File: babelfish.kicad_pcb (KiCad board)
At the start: 2 copper layers, 56 x 38.2 mm, 88 parts, among them J1 Conn_02x02_Odd_Even, J2 SWD, J3 DE9 Female, J4 USB_A, Q1 BSS138, SW1 TS342A2P-WZ, SW2 TS342A2P-WZ, SW3 SK12D07VG5_C3020419, U1 RP2040, U10 74HC4052PW,118, U11 MAX3232IDR, U2 TPS2113ADRBR, U3 GT-USB-7010ASV, U4 W25Q128JVS, U5 TPMCP1703T-5002E_CB, U6 TPMCP1703T-3302E_CB, U7 74HC4052PW,118, U8 74HC4052PW,118, U9 74HC4052PW,118, X1 X322512MSB4SI

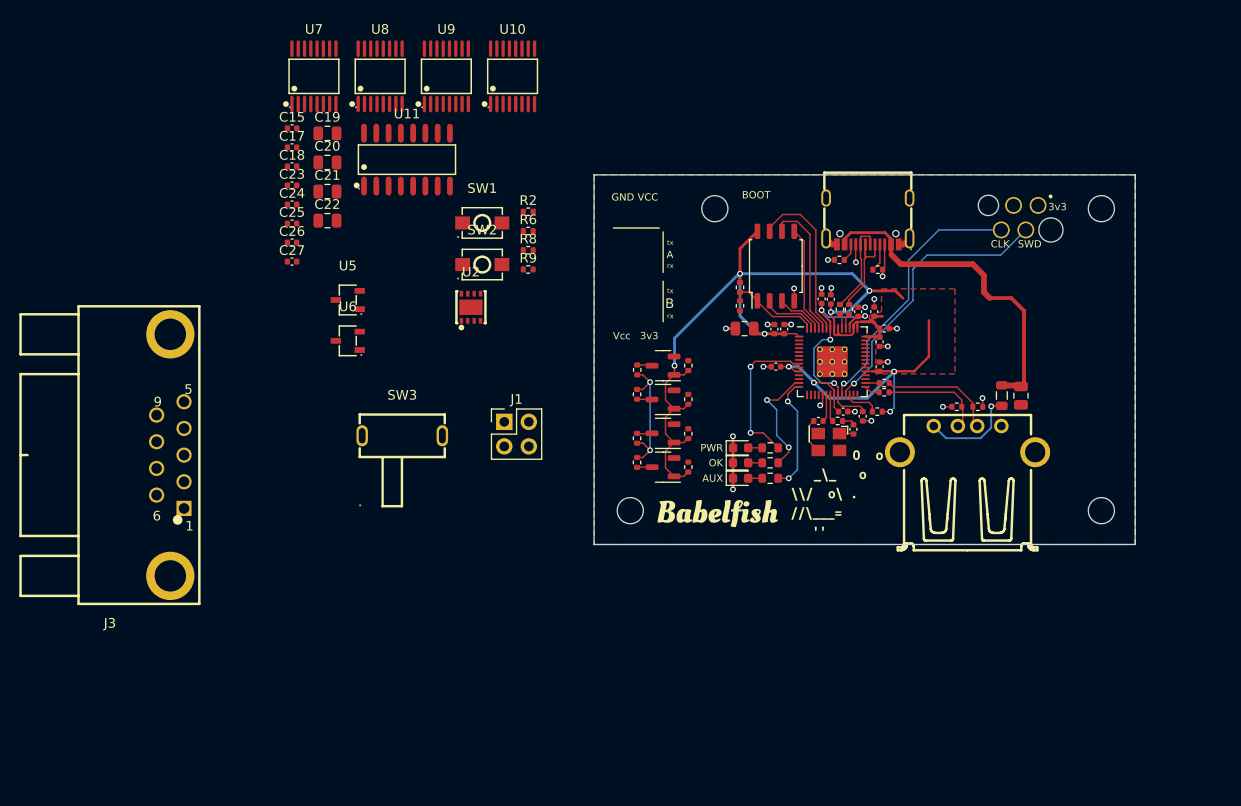
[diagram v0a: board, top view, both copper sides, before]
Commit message: Layout v2 done
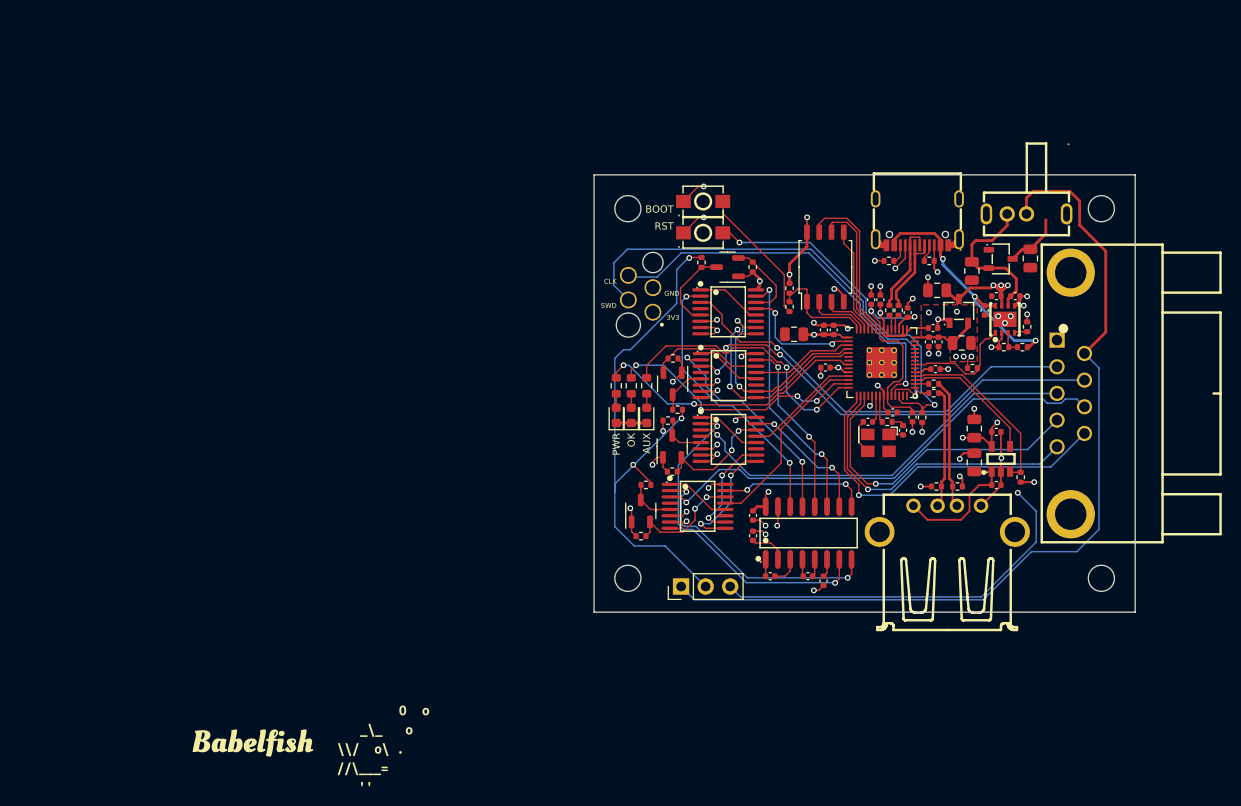
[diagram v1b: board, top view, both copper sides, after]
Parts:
- removed FB1: FerriteBead_Small, Inductor_SMD:L_0805_2012Metric
- added C29: 10u, Capacitor_SMD:C_0805_2012Metric, F.Cu at (121.6, 99.2)
- added C30: 100n, Capacitor_SMD:C_0402_1005Metric, F.Cu at (123.9, 96.1)
- added C31: 10u, Capacitor_SMD:C_0805_2012Metric, F.Cu at (121.6, 95.8)
- added R28: 10k, Resistor_SMD:R_0402_1005Metric, F.Cu at (126.4, 100.8)
- added U12: AP2191WG-7, lcsc:SOT-25-5_L2.9-W1.6-P0.95-LS2.8-BL, F.Cu at (124.4, 98.9)
- C28: value 10u -> 100n; footprint Capacitor_SMD:C_0805_2012Metric -> Capacitor_SMD:C_0402_1005Metric
- J1: value Conn_02x02_Odd_Even -> Shifter Power; footprint Connector_PinHeader_2.54mm:PinHeader_2x02_P2.54mm_Vertical -> Connector_PinHeader_2.54mm:PinHeader_1x03_P2.54mm_Vertical
- moved J3 93.4 mm to (131.6, 92.1), turned to 0 degrees
- moved C18 76.0 mm to (125.8, 82.1)
- moved C17 74.5 mm to (123.9, 82.1), turned to 180 degrees
- moved C15 74.1 mm to (122.7, 83.5), turned to -90 degrees
- moved C19 73.9 mm to (127.4, 78.2), turned to -90 degrees
- moved SW3 68.6 mm to (127.0, 73.5), turned to 180 degrees
- moved U5 67.7 mm to (124.3, 78.2), turned to 180 degrees
- moved C20 67.6 mm to (121.3, 79.5), turned to -90 degrees
- moved C22 66.9 mm to (120.3, 86.9)
- moved C27 64.2 mm to (106.0, 111.5), turned to -90 degrees
- moved C21 63.9 mm to (117.8, 81.5), turned to 180 degrees
- moved C26 63.6 mm to (104.4, 111.0)
- moved U6 63.3 mm to (120.0, 83.6), turned to -90 degrees
- moved C24 62.7 mm to (100.5, 111.0)
- moved C23 59.9 mm to (98.7, 106.8), turned to -90 degrees
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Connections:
- net Net-(U2-VSNS) renamed /PWR_VSNS
- C28 pad 1: VBUS -> /VBUS_OUT
- J1 pad 1: /5V0 -> /VCC_IN
- J1 pad 3: /VCC_IN -> /5V0
- J3 pad 2: /RX_A_CONN -> /TX_A_CONN
- J3 pad 3: /TX_A_CONN -> /TX_B_CONN
- J3 pad 4: unconnected-(J3-Pad4) -> /GPIO14
- J3 pad 5: unconnected-(J3-Pad5) -> /GPIO13
- J3 pad 7: /RX_B_CONN -> /RX_A_CONN
- J3 pad 8: /TX_B_CONN -> /RX_B_CONN
- J3 pad 9: unconnected-(J3-Pad9) -> /GPIO12
- J4 pad 1: Net-(J4-VBUS) -> /VBUS_OUT
- Q1 pad 2: /TX_A_1Y1 -> /RX_A_1Y1
- Q1 pad 3: /TX_A_2Y1 -> /RX_A_2Y1
- Q2 pad 2: /RX_A_1Y1 -> /TX_A_1Y1
- Q2 pad 3: /RX_A_2Y1 -> /TX_A_2Y1
- Q3 pad 3: /RX_B_2Y1 -> /TX_B_2Y1
- R18 pad 2: /TX_A_1Y1 -> /RX_A_1Y1
- R19 pad 2: /TX_A_2Y1 -> /RX_A_2Y1
- R20 pad 2: /RX_A_1Y1 -> /TX_A_1Y1
- R21 pad 2: /RX_A_2Y1 -> /TX_A_2Y1
- R23 pad 2: /RX_B_2Y1 -> /TX_B_2Y1
- U1 pad 15: /U0_TX_B -> /GPIO12
- U1 pad 16: /U0_RX_B -> /GPIO13
- U1 pad 31: /GPIO20 -> /USB2_EN
- U1 pad 32: /GPIO21 -> /USB2_FLG
- U1 pad 35: /GPIO23 -> /STAT_5V0
- U1 pad 4: /GPIO2 -> /CH_A_S0
- U1 pad 5: /GPIO3 -> /CH_A_S1
- U10 pad 1: /RX_B_2Y0 -> /RX_B_Y0_THRU
- U10 pad 12: /RX_B_1Y0 -> /RX_B_Y0_THRU
- U10 pad 13: /RX_A -> /RX_B
- U11 pad 7: /RX_B_1Y2 -> /TX_B_2Y2
- U11 pad 8: /TX_B_2Y2 -> /RX_B_2Y2
- U7 pad 1: /TX_A_2Y0 -> /TX_A_Y0_THRU
- U7 pad 12: /TX_A_1Y0 -> /TX_A_Y0_THRU
- U8 pad 1: /RX_A_2Y0 -> /RX_A_Y0_THRU
- U8 pad 12: /RX_A_1Y0 -> /RX_A_Y0_THRU
- U9 pad 1: /TX_B_2Y0 -> /TX_B_Y0_THRU
- U9 pad 12: /TX_B_1Y0 -> /TX_B_Y0_THRU
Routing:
- net /VCC_IN: track 0.00 -> 91.3 mm
- net +3V3: track 125.6 -> 62.2 mm, vias 9 -> 21
- net /5V0: track 0.00 -> 59.0 mm, vias 0 -> 6
- net GND: track 42.4 -> 98.8 mm, vias 22 -> 43
- net /RX_B_CONN: track 0.00 -> 49.0 mm, vias 0 -> 1
- net /VSHIFT: track 13.7 -> 60.7 mm, vias 2 -> 4
- net /RX_A_CONN: track 0.00 -> 46.5 mm, vias 0 -> 3
- net /TX_A_CONN: track 0.00 -> 44.0 mm, vias 0 -> 1
- net /TX_B_CONN: track 0.00 -> 42.8 mm, vias 0 -> 1
- net /GPIO12: track 0.00 -> 37.4 mm, vias 0 -> 1
- net /TX_B_2Y2: track 0.00 -> 35.0 mm, vias 0 -> 2
- net /RUN: track 3.67 -> 38.1 mm, vias 0 -> 2
- net /GPIO14: track 0.00 -> 32.9 mm, vias 0 -> 1
- net /GPIO13: track 0.00 -> 32.5 mm, vias 0 -> 1
- net /TX_A_2Y2: track 0.00 -> 28.8 mm, vias 0 -> 2
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- added copper zone on In2.Cu, net +3V3
- added copper zone on In2.Cu, net /5V0
- added copper zone on In1.Cu, net GND
- removed copper zone on B.Cu, net GND
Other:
- board size 56 x 38.2 mm -> 56 x 45.2 mm
- copper layers 2 -> 4
- board text added: "3V3"
- board text added: "RST"
- board text removed: "3v3"
- board text removed: "A"
- board text removed: "B"
- board text removed: "VCC"
- board text removed: "Vcc"
- board text removed: "rx"
- board text removed: "tx"
